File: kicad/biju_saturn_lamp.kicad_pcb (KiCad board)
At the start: 2 copper layers, 82.3 x 59.9 mm, 25 parts, among them J1 Barrel_Jack, J2 Conn_01x06, J3 Conn_01x02, J4 Conn_01x02, J5 Conn_01x02, SW1 SW_Push, U1 Pico, U2 74HC595, U3 PAM8302AAD

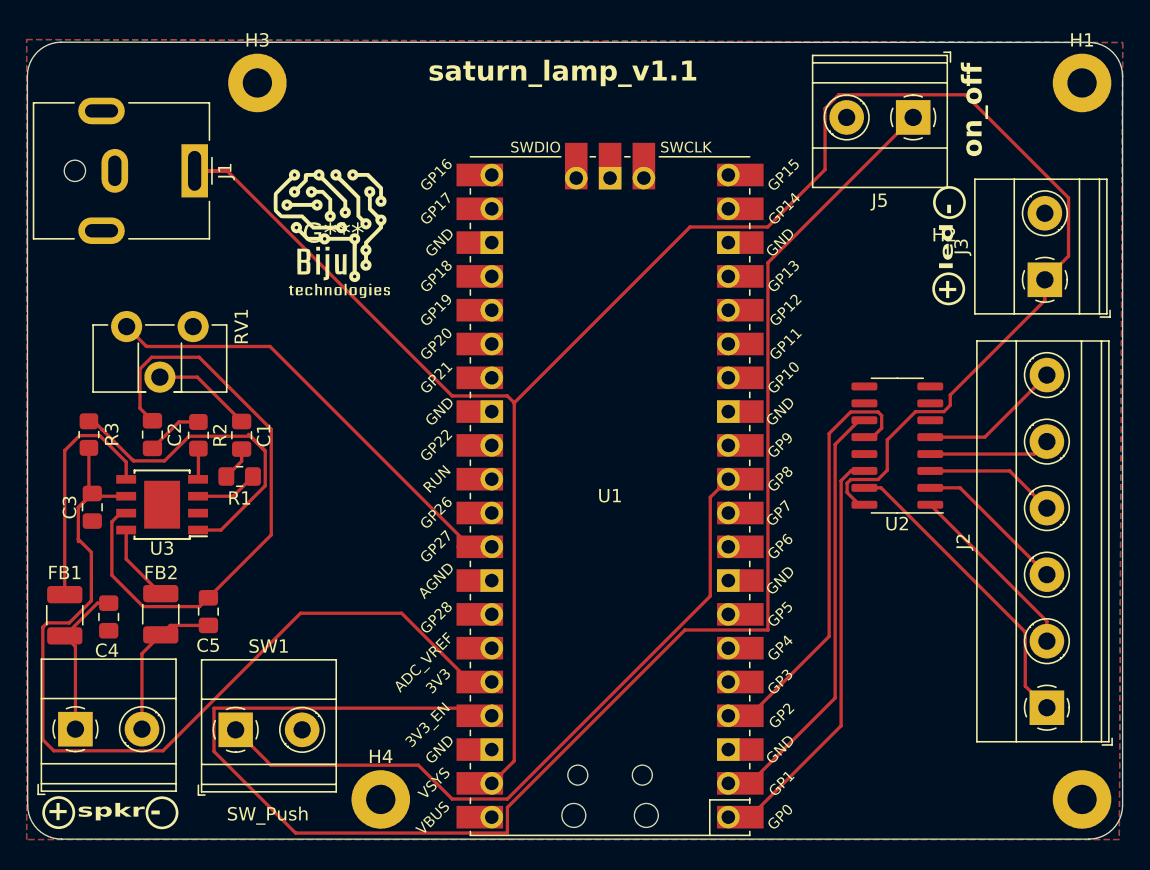
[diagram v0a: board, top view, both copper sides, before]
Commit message: update pcb
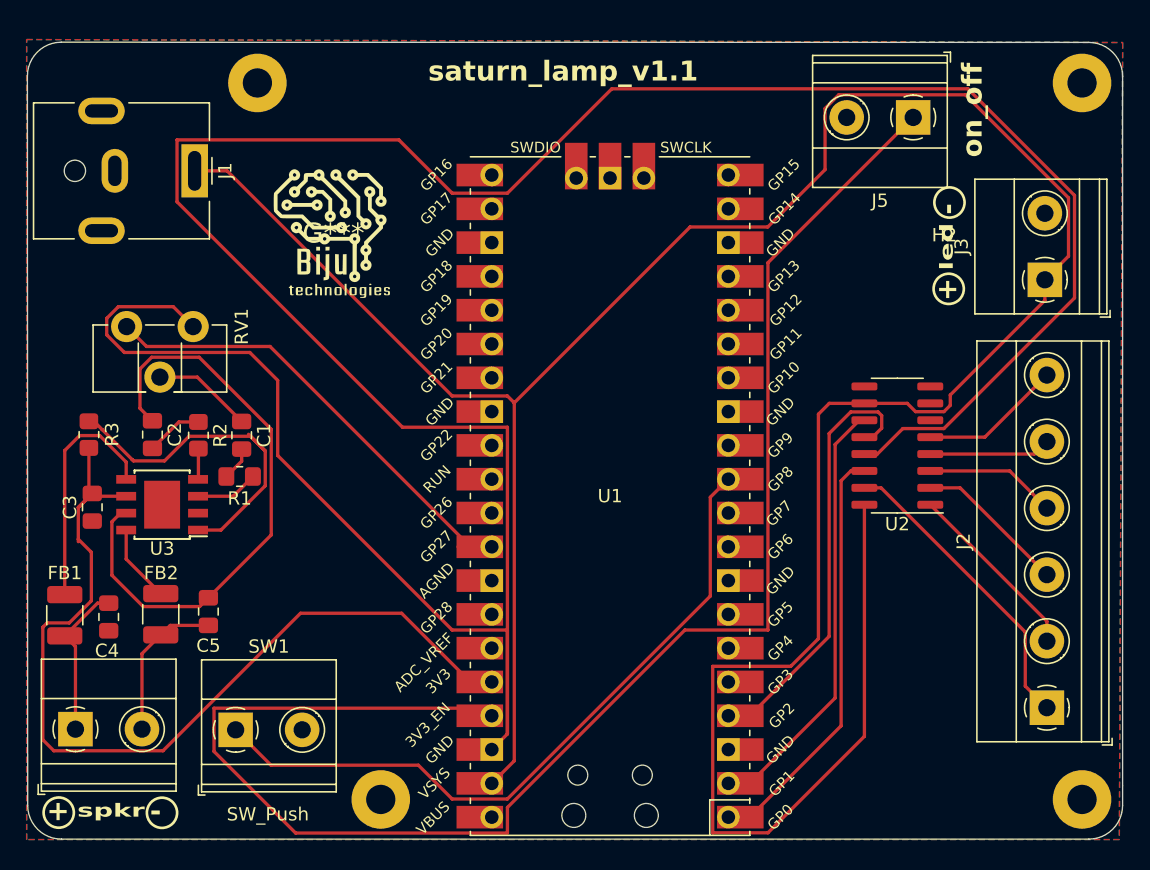
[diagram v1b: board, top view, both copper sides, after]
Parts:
- C4, C5: value 220uF -> 220nF
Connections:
- U2 pad 10: unconnected-(U2-~{SRCLR}-Pad10) -> VCC
- U2 pad 13: unconnected-(U2-~{OE}-Pad13) -> GND
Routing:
- net GND: track 45.4 -> 269.8 mm
- net VCC: track 153.5 -> 218.0 mm
